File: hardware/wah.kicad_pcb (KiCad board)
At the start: 4 copper layers, 99.1 x 54.5 mm, 34 parts, among them J1 Barrel_Jack_Switch, J2 In, J3 Out, SW1 SW_Push_3PDT, U1 TL072, U2 L78L05_TO92

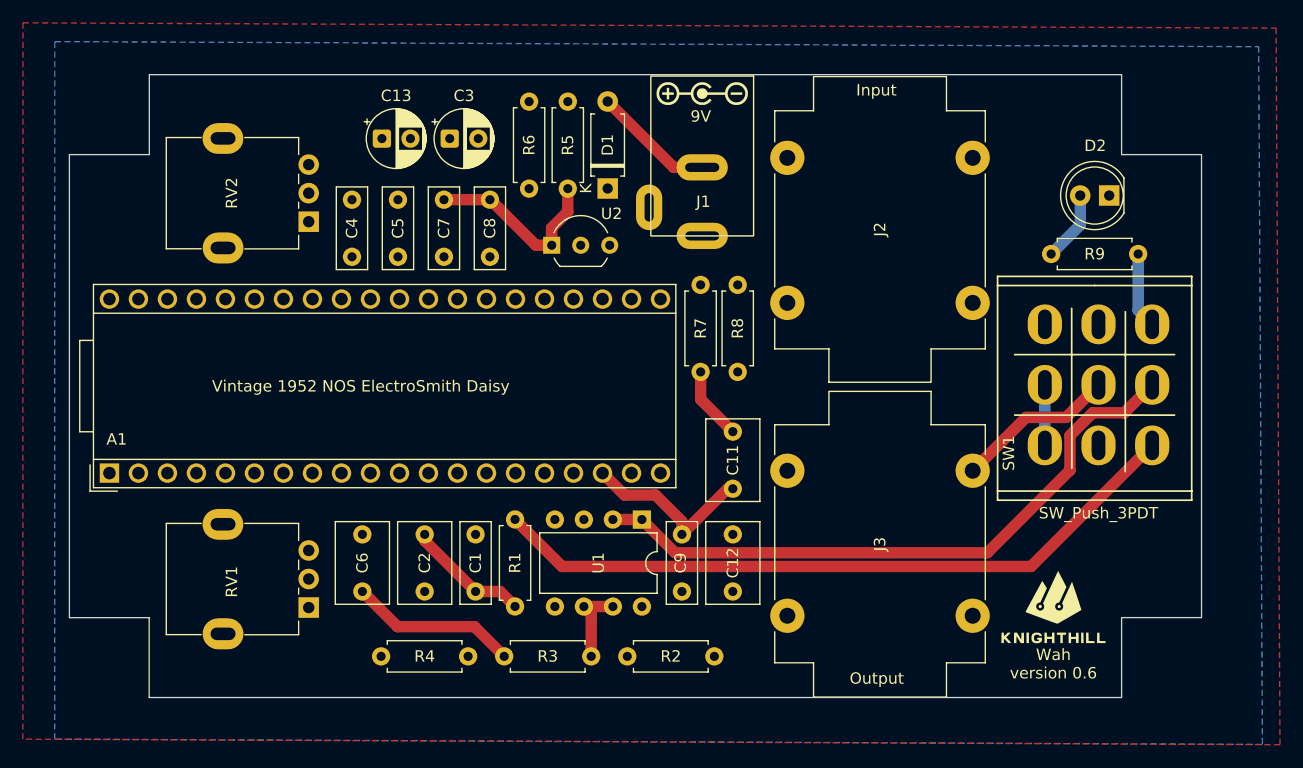
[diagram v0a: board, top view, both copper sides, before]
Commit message: rearrange pcb
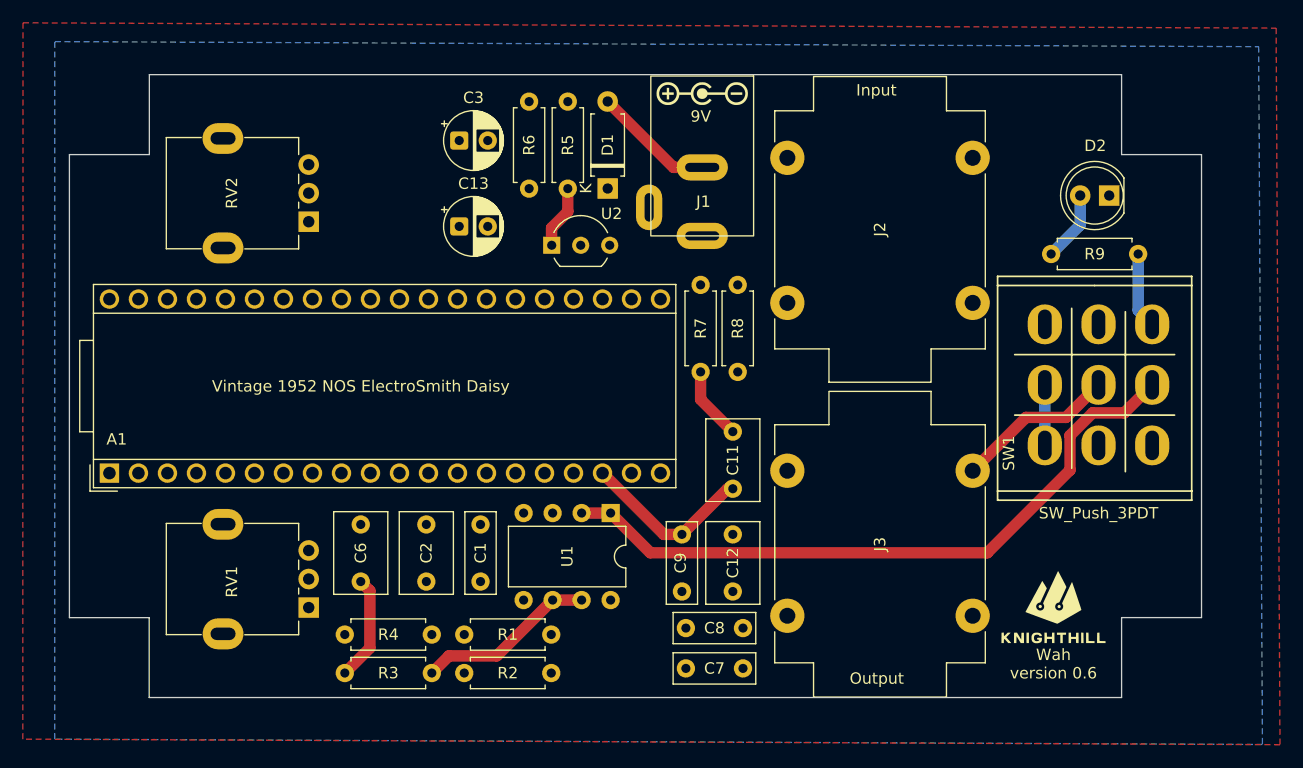
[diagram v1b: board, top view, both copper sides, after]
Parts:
- removed C4, C5: 100n, Capacitor_THT:C_Rect_L7.0mm_W2.5mm_P5.00mm
- moved C7 46.2 mm to (96.4, 85.2), turned to 0 degrees
- moved C8 41.3 mm to (96.4, 81.6), turned to 0 degrees
- moved R2 14.4 mm to (84.6, 85.6)
- moved R3 14.0 mm to (74.2, 85.6)
- moved R1 10.6 mm to (84.6, 82.2), turned to 180 degrees
- moved C13 10.2 mm to (76.5, 46.5)
- moved R4 3.71 mm to (66.5, 82.2)
- moved U1 2.80 mm to (89.8, 71.6)
- moved C1 0.97 mm to (78.4, 77.6)
- moved C2 0.88 mm to (73.7, 72.6)
- moved C6 0.88 mm to (67.9, 77.6)
- moved C3 0.85 mm to (76.5, 39.0)
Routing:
- net Net-(U1B--): track 7.17 -> 15.8 mm
- net Net-(C6-Pad1): track 14.8 -> 9.25 mm
- net Net-(U1B-+): track 21.3 -> 17.7 mm
- net /FX_OUT: track 56.3 -> 59.3 mm
- net Net-(U1A-+): track 39.1 -> 42.1 mm
- net /AUDIO_IN: track 30.8 -> 28.8 mm
- net /FX_IN: track 61.9 -> 60.3 mm
- net Net-(C1-Pad1): track 10.8 -> 12.2 mm
- net /AUDIO_OUT: track 16.0 -> 15.3 mm
- net Net-(U1C-V+): track 58.3 -> 58.9 mm
